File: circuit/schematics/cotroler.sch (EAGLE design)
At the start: 17 parts

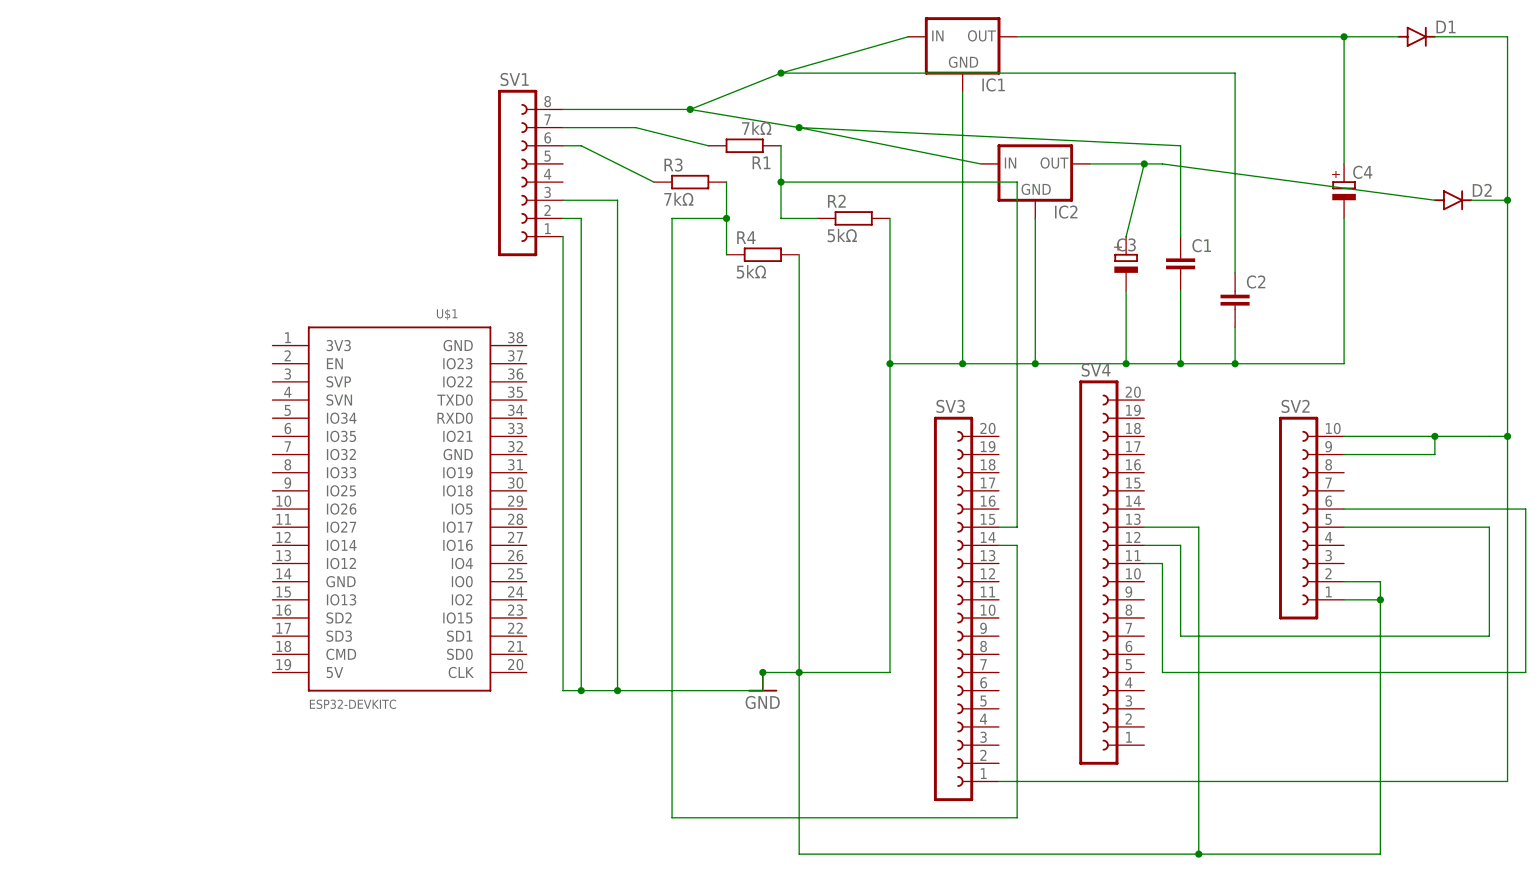
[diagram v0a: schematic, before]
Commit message: dekita
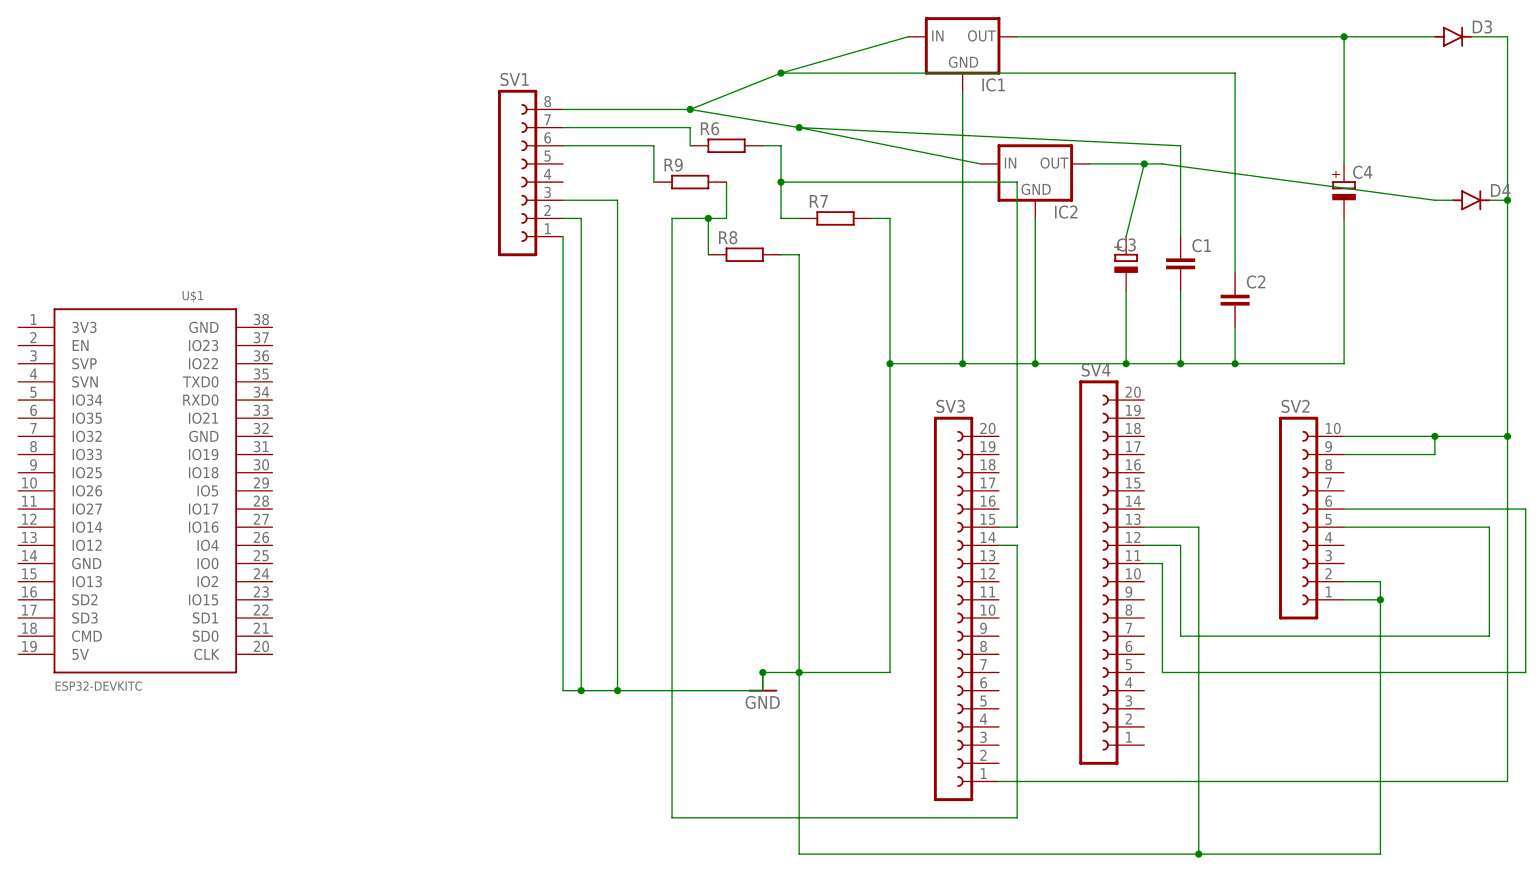
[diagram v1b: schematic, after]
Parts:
- removed D1, D2: (no value), diode:DIODE-C1702-15
- removed R1, R3: 7kΩ, rcl:R-EU_0204/2V
- removed R2, R4: 5kΩ, rcl:R-EU_0204/2V
- added D3, D4: (no value), diode:DIODE-D-10
- added R6, R7, R8, R9: (no value), resistor:R-EU_0207/10
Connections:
- net GND: now also R7.2, R8.2; no longer R2.2, R4.2
- net N$1: now also R6.1; no longer R1.2
- net N$10: now also D3.C, D4.C; no longer D1.C, D2.C
- net N$4: now also R6.2, R7.1; no longer R1.1, R2.1
- net N$5: now also R9.1; no longer R3.1
- net N$6: now also R8.1, R9.2; no longer R3.2, R4.1
- net N$7: now also D4.A; no longer D2.A
- net N$8: now also D3.A; no longer D1.A
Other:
- moved on the sheet: U$1
